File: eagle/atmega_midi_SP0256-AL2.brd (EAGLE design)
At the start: 100 x 80 mm, 42 parts, among them U1 6N138, U2 ATMEGA328P_PDIP, U3 SP0256-AL2, U4 TL072P

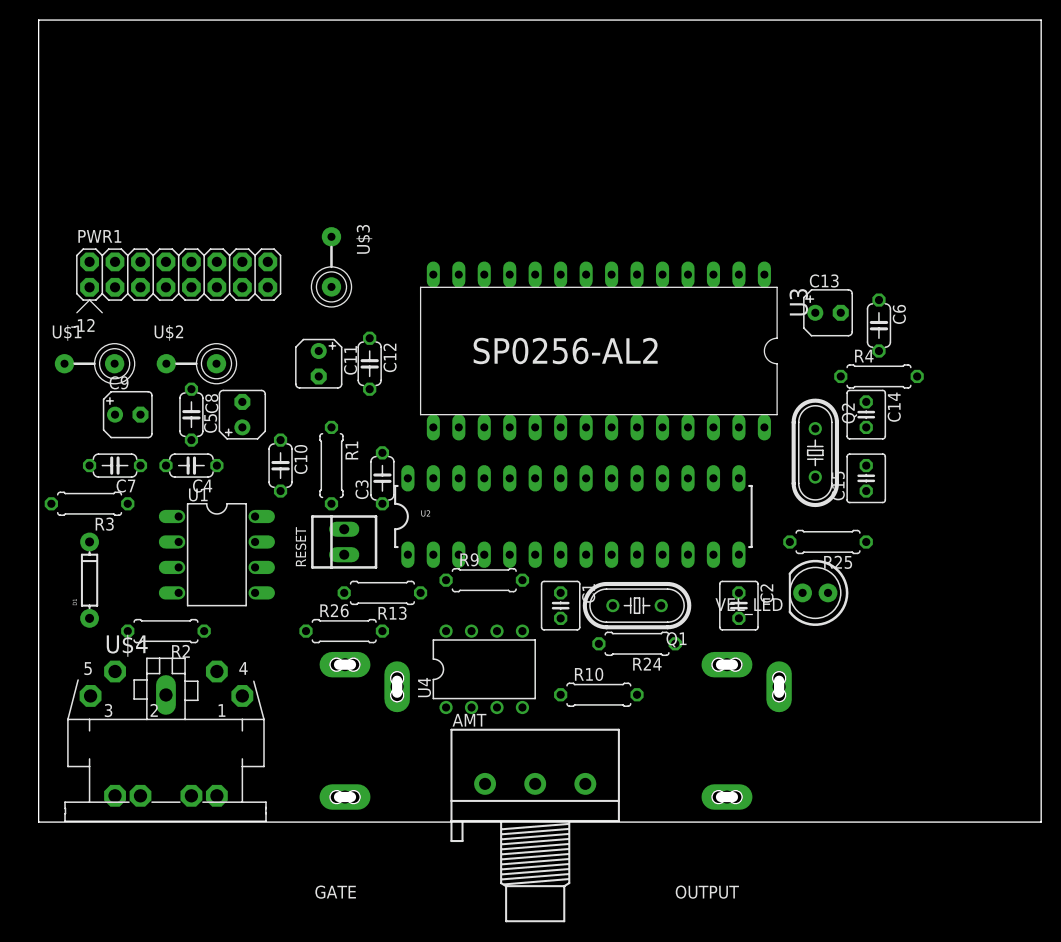
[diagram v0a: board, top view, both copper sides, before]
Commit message: layout adjusting
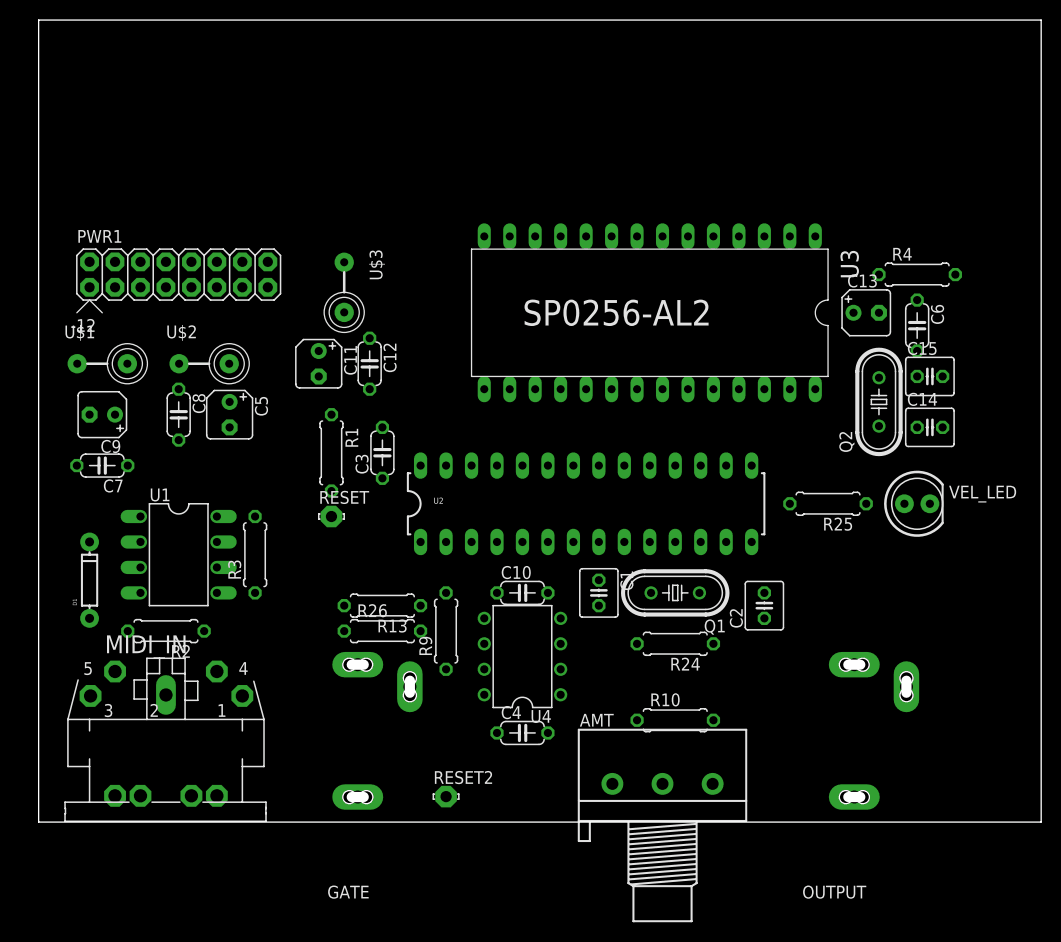
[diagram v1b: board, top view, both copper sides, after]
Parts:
- added RESET2: LSP11, solpad:LSP11
- RESET: value 22-23-2021 -> LSP11; device con-molex:22-23-2021 -> solpad:LSP11
- moved C4 42.4 mm to (48.3, 8.89), turned to 0 degrees
- moved C10 27.3 mm to (48.3, 22.9), turned to 0 degrees
- moved R3 17.3 mm to (21.6, 26.7), turned to 90 degrees
- moved VEL_LED 13.5 mm to (87.6, 31.8), turned to 0 degrees
- moved OUTPUT 12.7 mm to (86.4, 0.00)
- moved AMT 12.7 mm to (62.2, 3.81)
- moved C15 12.0 mm to (88.9, 44.5), turned to 0 degrees
- moved R4 10.9 mm to (87.6, 54.6)
- moved Q2 8.13 mm to (83.8, 41.9), turned to 90 degrees
- moved R10 8.03 mm to (63.5, 10.2)
- moved C14 6.48 mm to (88.9, 39.4), turned to 0 degrees
- moved R9 6.35 mm to (40.6, 19.1), turned to 90 degrees
- moved U3 6.35 mm to (61.0, 50.8)
- moved C1 4.02 mm to (55.9, 22.9)
- moved Q1 4.02 mm to (63.5, 22.9)
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- renumbered U$4 to MIDI_IN
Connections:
- net GND: now also MIDI_IN.PE, MIDI_IN.PE1, MIDI_IN.PE2, MIDI_IN.PE@
- net N$15: now also U2.18, U3.P$20; no longer U2.5, U3.P$19
- net N$27: now also U2.19, U3.P$19; no longer U2.4, U3.P$20
- net N$28: now also U2.15; no longer U2.18
- net N$29: now also RESET2.MP; no longer RESET.2
- net N$43: now also RESET.MP; no longer RESET.1

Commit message: 93pct auto
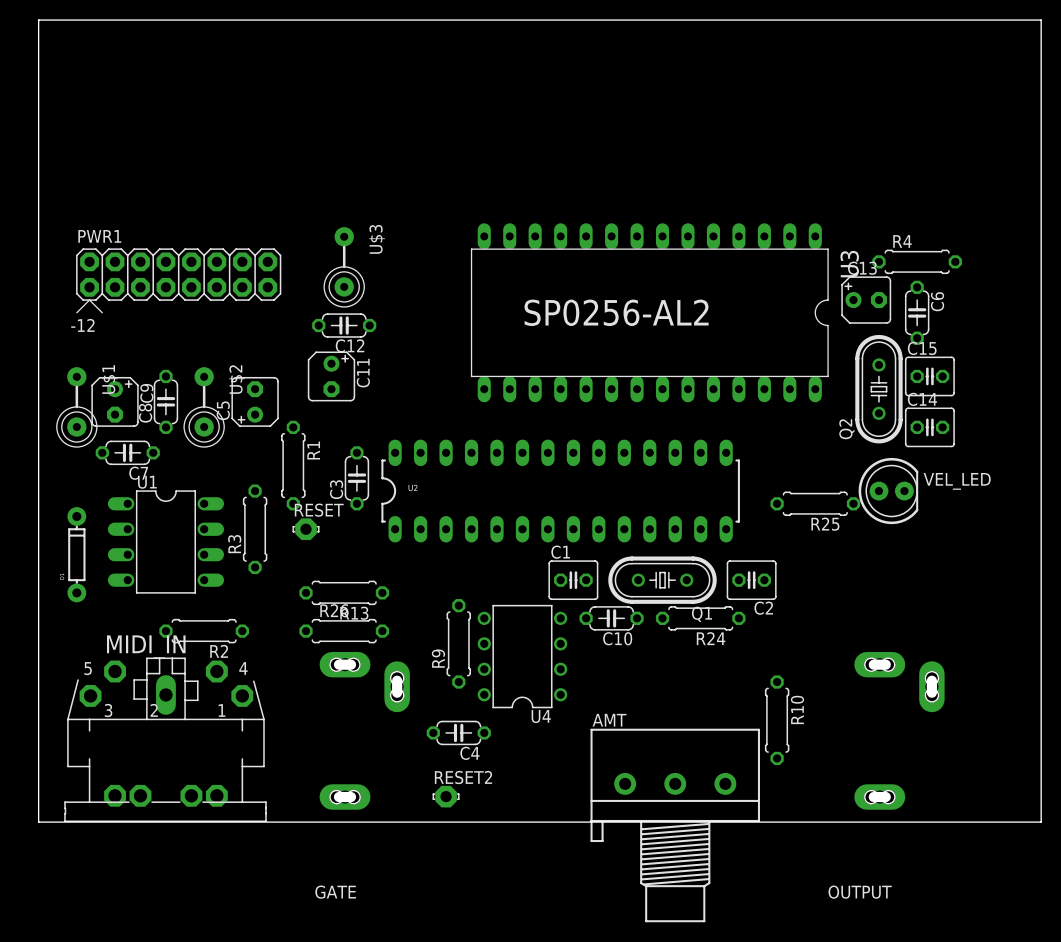
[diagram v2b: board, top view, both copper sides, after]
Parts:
- moved R10 10.2 mm to (73.7, 10.2), turned to 270 degrees
- moved C10 9.25 mm to (57.1, 20.3), turned to 180 degrees
- moved C4 6.35 mm to (41.9, 8.89), turned to 180 degrees
- moved C12 4.58 mm to (30.5, 49.5), turned to 180 degrees
- moved U$1 4.58 mm to (3.81, 41.9), turned to 270 degrees
- moved R1 4.02 mm to (25.4, 35.6)
- moved R13 4.02 mm to (30.5, 22.9)
- moved R2 3.81 mm to (16.5, 19.1)
- moved U$2 3.81 mm to (16.5, 41.9), turned to 270 degrees
- moved R26 3.81 mm to (30.5, 19.1)
- moved R24 3.59 mm to (66.0, 20.3)
- moved C3 3.59 mm to (31.8, 34.3)
- moved D1 2.84 mm to (3.81, 26.7)
- moved U2 2.84 mm to (52.1, 33.0)
- moved C1 2.84 mm to (53.3, 24.1), turned to 0 degrees
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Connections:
- removed net N$1: C4.2, C7.1
- net GND: now also C4.2, C7.1, GATE.P$1, OUTPUT.P$1, R13.2, RESET2.MP, U1.5
- net N$28: now also U2.17; no longer U2.15
- net N$29: no longer GATE.P$1, OUTPUT.P$1, R13.2, RESET2.MP, U1.5

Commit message: routed
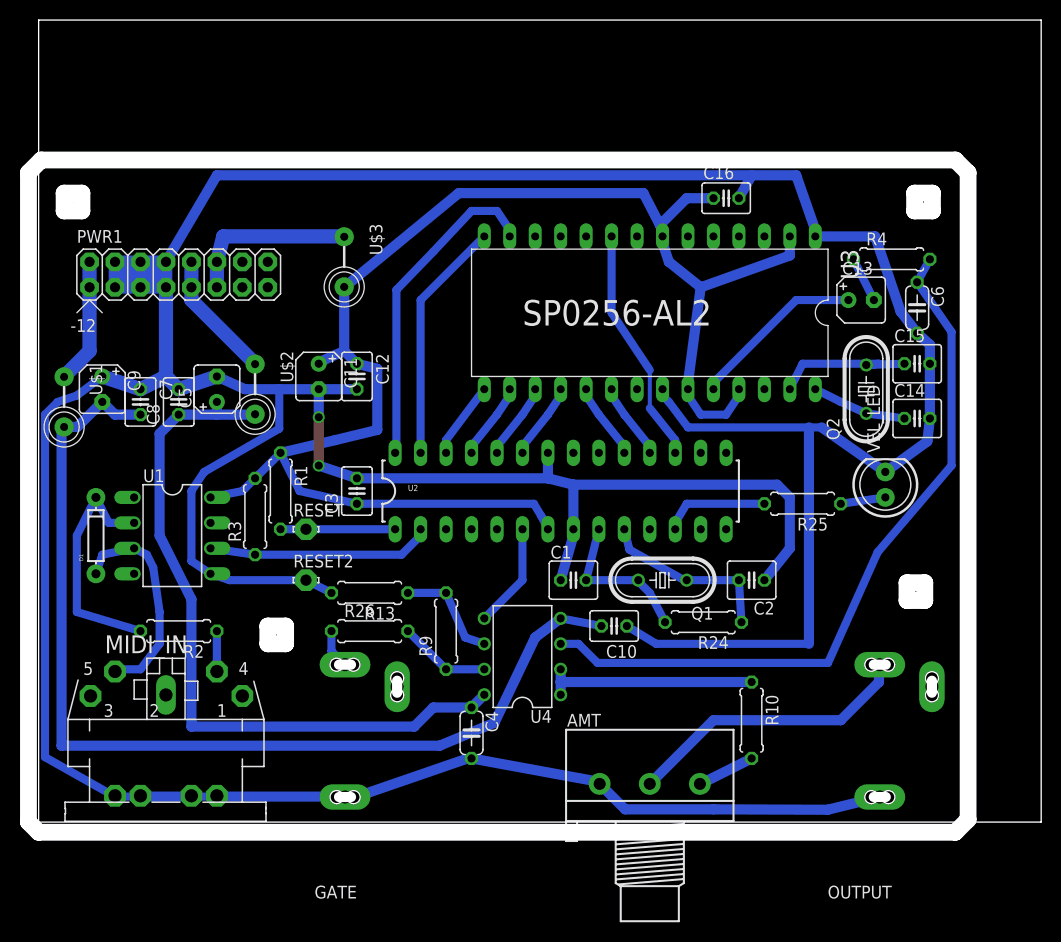
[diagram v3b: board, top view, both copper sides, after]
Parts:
- added C16: 100n, rcl:C025-030X050
- C10, C12, C3, C7, C8: device rcl:C050-024X044 -> rcl:C025-030X050
- moved RESET2 25.7 mm to (26.7, 24.1)
- moved U$2 5.24 mm to (21.6, 43.2)
- moved C12 5.24 mm to (31.8, 44.5), turned to 270 degrees
- moved C7 5.24 mm to (10.2, 41.9), turned to 270 degrees
- moved C5 4.02 mm to (17.8, 43.2)
- moved R1 2.84 mm to (24.1, 33.0)
- moved D1 2.69 mm to (5.71, 28.6)
- moved R4 2.55 mm to (85.1, 56.1)
- moved R13 2.54 mm to (33.0, 22.9)
- moved R26 2.54 mm to (33.0, 19.1)
- moved R2 2.54 mm to (14.0, 19.1)
- moved AMT 2.54 mm to (61.0, 3.81)
- moved R10 2.54 mm to (71.1, 10.2)
- moved C15 1.80 mm to (87.6, 45.7)
- moved C9 1.80 mm to (6.35, 43.2)
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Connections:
- removed net N$29: C1.1, C10.1, C11.-, C12.2, C2.1, C3.2, C5.-, C8.2, C9.+, PWR1.3, PWR1.4, PWR1.5, PWR1.6, PWR1.7, PWR1.8, U2.22, U2.8
- net +5V: now also C16.1
- net GND: now also C1.1, C10.1, C11.-, C12.2, C16.2, C2.1, C3.2, C5.-, C8.2, C9.+, PWR1.3, PWR1.4, PWR1.5, PWR1.6, PWR1.7, PWR1.8, U2.22, U2.8
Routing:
- net GND: track 0.00 -> 469.7 mm, vias 0 -> 2
- net +5V: track 0.00 -> 149.7 mm
- net -12V: track 0.00 -> 101.6 mm
- net N$6: track 0.00 -> 72.9 mm
- net +12V: track 0.00 -> 72.1 mm
- net N$26: track 0.00 -> 32.6 mm
- net N$13: track 0.00 -> 28.8 mm
- net N$25: track 0.00 -> 24.2 mm
- net N$7: track 0.00 -> 23.9 mm
- net N$28: track 0.00 -> 23.6 mm
- net N$30: track 0.00 -> 22.4 mm
- net N$3: track 0.00 -> 21.7 mm
- net N$12: track 0.00 -> 21.6 mm
- net N$5: track 0.00 -> 18.0 mm
- net N$17: track 0.00 -> 17.5 mm
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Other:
- board size 100 x 80 mm -> 101 x 81 mm
